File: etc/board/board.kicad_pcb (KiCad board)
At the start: 2 copper layers, 152.2 x 109.4 mm, 10 parts, among them J1 Conn_01x05, U1 Teensy4.1, U2 BOB-09056, U3 TFT_320x240

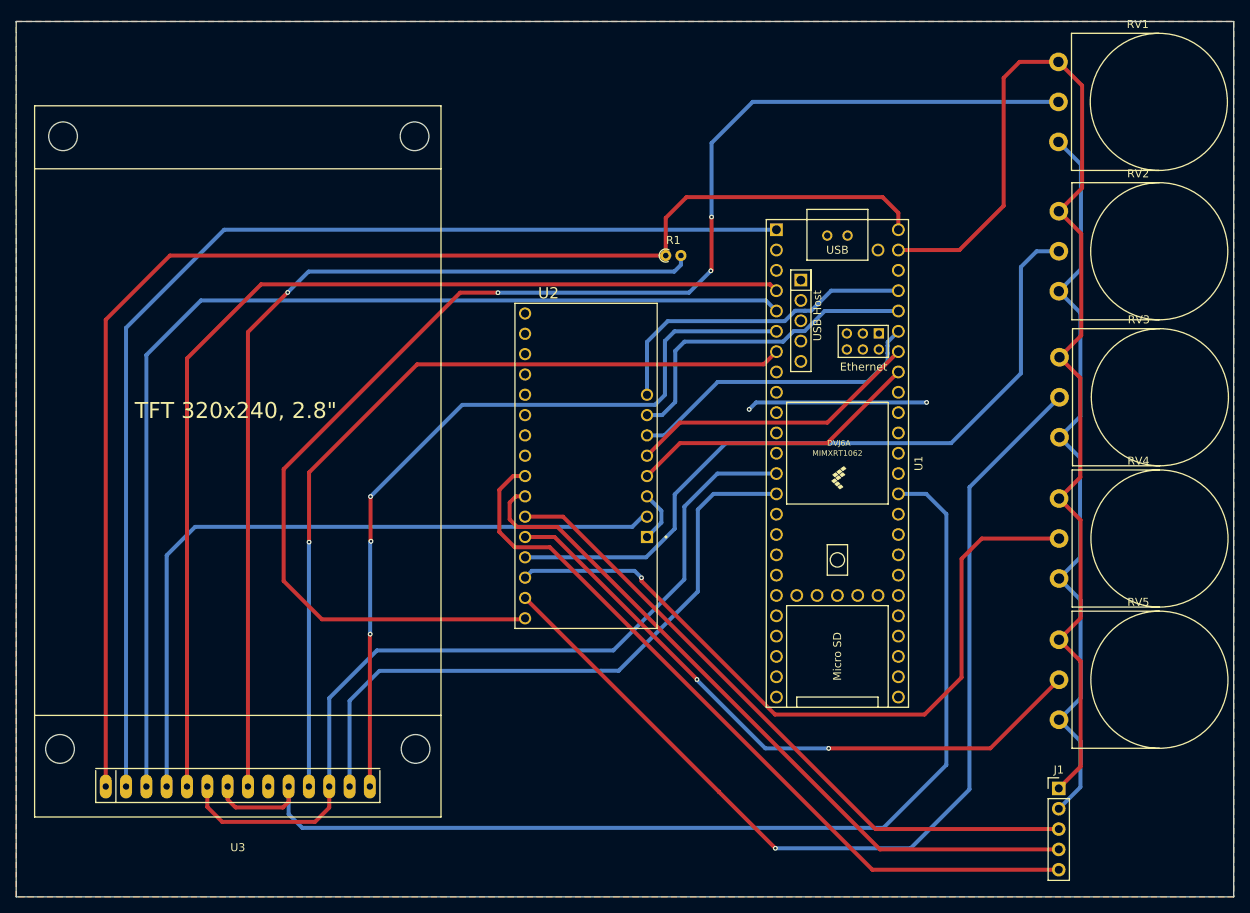
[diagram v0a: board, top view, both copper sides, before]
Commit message: Update code for board v2
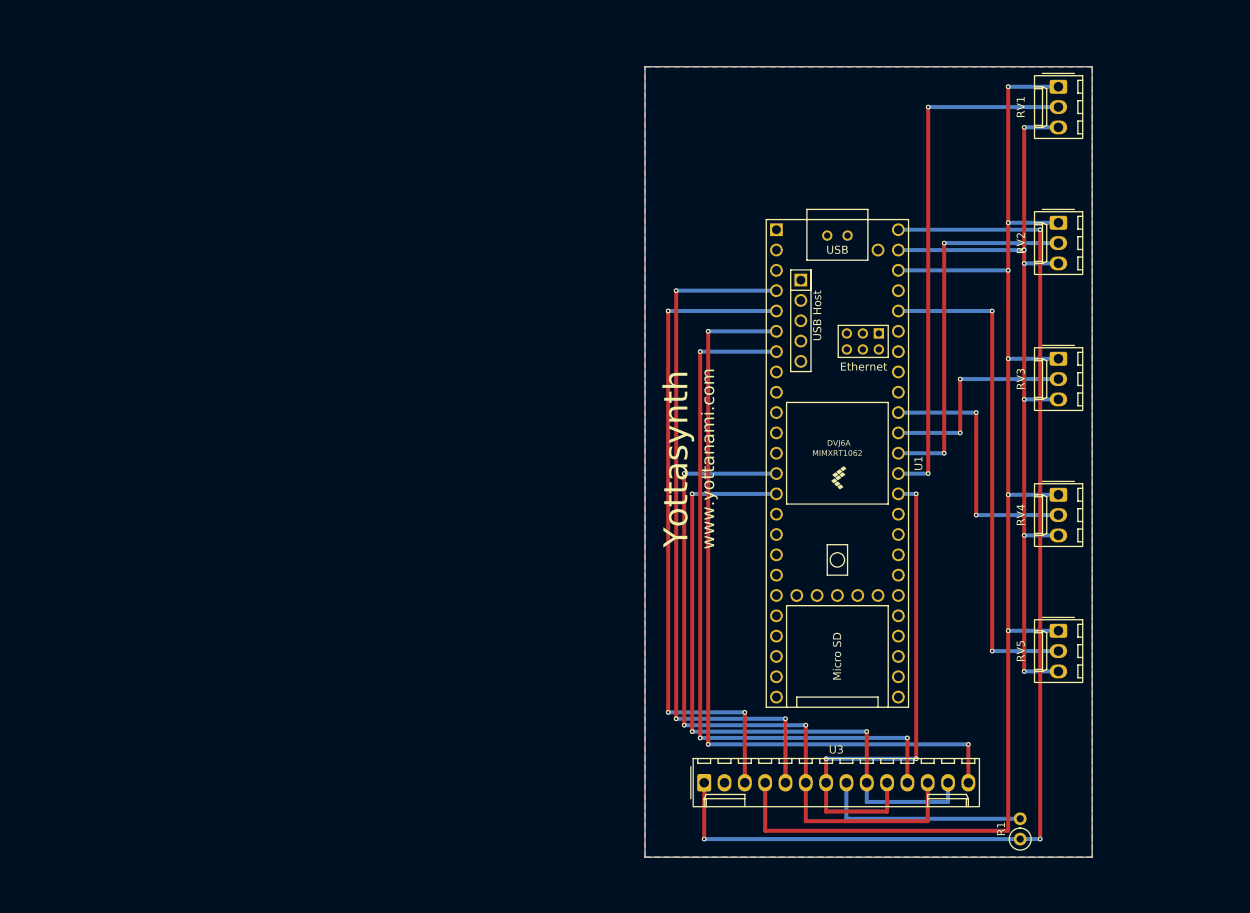
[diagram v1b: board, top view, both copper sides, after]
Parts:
- removed J1: Conn_01x05, Connector_PinHeader_2.54mm:PinHeader_1x05_P2.54mm_Vertical
- removed U2: BOB-09056, BOB-09056:MODULE_BOB-09056
- R1: footprint Resistor_THT:R_Axial_DIN0204_L3.6mm_D1.6mm_P1.90mm_Vertical -> Resistor_THT:R_Axial_DIN0207_L6.3mm_D2.5mm_P2.54mm_Vertical
- RV1, RV2, RV3, RV4, RV5: footprint Potentiometer_THT:Potentiometer_Omeg_PC16BU_Vertical -> Connector_Molex:Molex_KK-254_AE-6410-03A_1x03_P2.54mm_Vertical
- U3: footprint TFT:TFT-320x240 -> Connector_Molex:Molex_KK-254_AE-6410-14A_1x14_P2.54mm_Vertical
- moved R1 85.3 mm to (220.5, 134.0), turned to 90 degrees
- moved U3 58.3 mm to (181.0, 127.0)
- moved RV5 11.1 mm to (225.3, 108.0), turned to -90 degrees
- moved RV4 10.5 mm to (225.3, 91.0), turned to -90 degrees
- moved RV3 9.81 mm to (225.3, 74.0), turned to -90 degrees
- moved RV2 8.56 mm to (225.3, 57.0), turned to -90 degrees
- moved RV1 6.89 mm to (225.3, 40.0), turned to -90 degrees
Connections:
- RV1 pad 2: Net-(U2-C0) -> /POT1
- RV2 pad 2: Net-(U2-C3) -> /POT2
- RV3 pad 2: Net-(U2-C1) -> /POT3
- RV4 pad 2: Net-(U2-C2) -> /POT4
- RV5 pad 2: Net-(U2-C4) -> /POT5
- U1 pad 14: Net-(U1-12_MISO_MQSL) -> /MISO
- U1 pad 15: unconnected-(U1-3V3-Pad15) -> /3V3
- U1 pad 36: unconnected-(U1-14_A0_TX3_SPDIF_OUT-Pad36) -> /POT1
- U1 pad 37: unconnected-(U1-15_A1_RX3_SPDIF_IN-Pad37) -> /POT2
- U1 pad 38: unconnected-(U1-16_A2_RX4_SCL1-Pad38) -> /POT3
- U1 pad 39: unconnected-(U1-17_A3_TX4_SDA1-Pad39) -> /POT4
- U1 pad 41: Net-(U1-19_A5_SCL) -> unconnected-(U1-19_A5_SCL-Pad41)
- U1 pad 42: Net-(U1-20_A6_TX5_LRCLK1) -> unconnected-(U1-20_A6_TX5_LRCLK1-Pad42)
- U1 pad 43: Net-(U1-21_A7_RX5_BCLK1) -> unconnected-(U1-21_A7_RX5_BCLK1-Pad43)
- U1 pad 44: Net-(U1-22_A8_CTX1) -> /POT5
- U1 pad 45: Net-(U1-23_A9_CRX1_MCLK1) -> unconnected-(U1-23_A9_CRX1_MCLK1-Pad45)
- U3 pad 13: Net-(U1-12_MISO_MQSL) -> /MISO
- U3 pad 9: unconnected-(U3-MISO-Pad9) -> /MISO
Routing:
- net GND: track 314.1 -> 105.1 mm, vias 2 -> 6
- net Net-(U2-C0): track 171.4 -> 0.00 mm, vias 3 -> 0
- net Net-(U2-C1): track 125.2 -> 0.00 mm, vias 1 -> 0
- net Net-(J1-Pin_5): track 96.6 -> 0.00 mm
- net Net-(U2-C3): track 92.9 -> 0.00 mm
- net Net-(U2-C2): track 92.6 -> 0.00 mm, vias 1 -> 0
- net Net-(J1-Pin_4): track 90.1 -> 0.00 mm
- net Net-(U3-LED): track 115.6 -> 26.2 mm, vias 1 -> 0
- net /MISO: track 0.00 -> 83.4 mm, vias 0 -> 3
- net Net-(J1-Pin_3): track 82.9 -> 0.00 mm
- net Net-(U2-C4): track 81.3 -> 0.00 mm, vias 2 -> 0
- net Net-(U1-12_MISO_MQSL): track 80.8 -> 0.00 mm
- net Net-(U1-13_SCK_LED): track 139.9 -> 64.4 mm, vias 0 -> 3
- net /POT1: track 0.00 -> 65.8 mm, vias 0 -> 2
- net /POT5: track 0.00 -> 62.5 mm, vias 0 -> 2
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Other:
- board size 152.2 x 109.4 mm -> 55.9 x 98.8 mm
- board text added: "Yottasynth"
- board text added: "www.yottanami.com"
